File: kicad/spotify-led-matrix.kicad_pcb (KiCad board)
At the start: 2 copper layers, 101.5 x 128 mm, 73 parts, among them J1 +5V, J6 USB_C_Receptacle_USB2.0, Q1 IRLML6244TRPBF, Q10 IRLML6244TRPBF, Q2 SS8050-G, Q3 SS8050-G, Q4 IRLML6244TRPBF, Q5 IRLML6244TRPBF, Q6 IRLML6244TRPBF, Q7 IRLML6244TRPBF, Q8 IRLML6244TRPBF, Q9 IRLML6244TRPBF, SW1 SELECT, SW2 EN, SW3 BOOT, U1 ESP32-WROOM-32E, U2 5V_TO_3V3, U3 MC74HC1G14DTT1G, U6 MC74HC1G14DTT1G, U7 MC74HC1G14DTT1G, U8 FT234XD-R

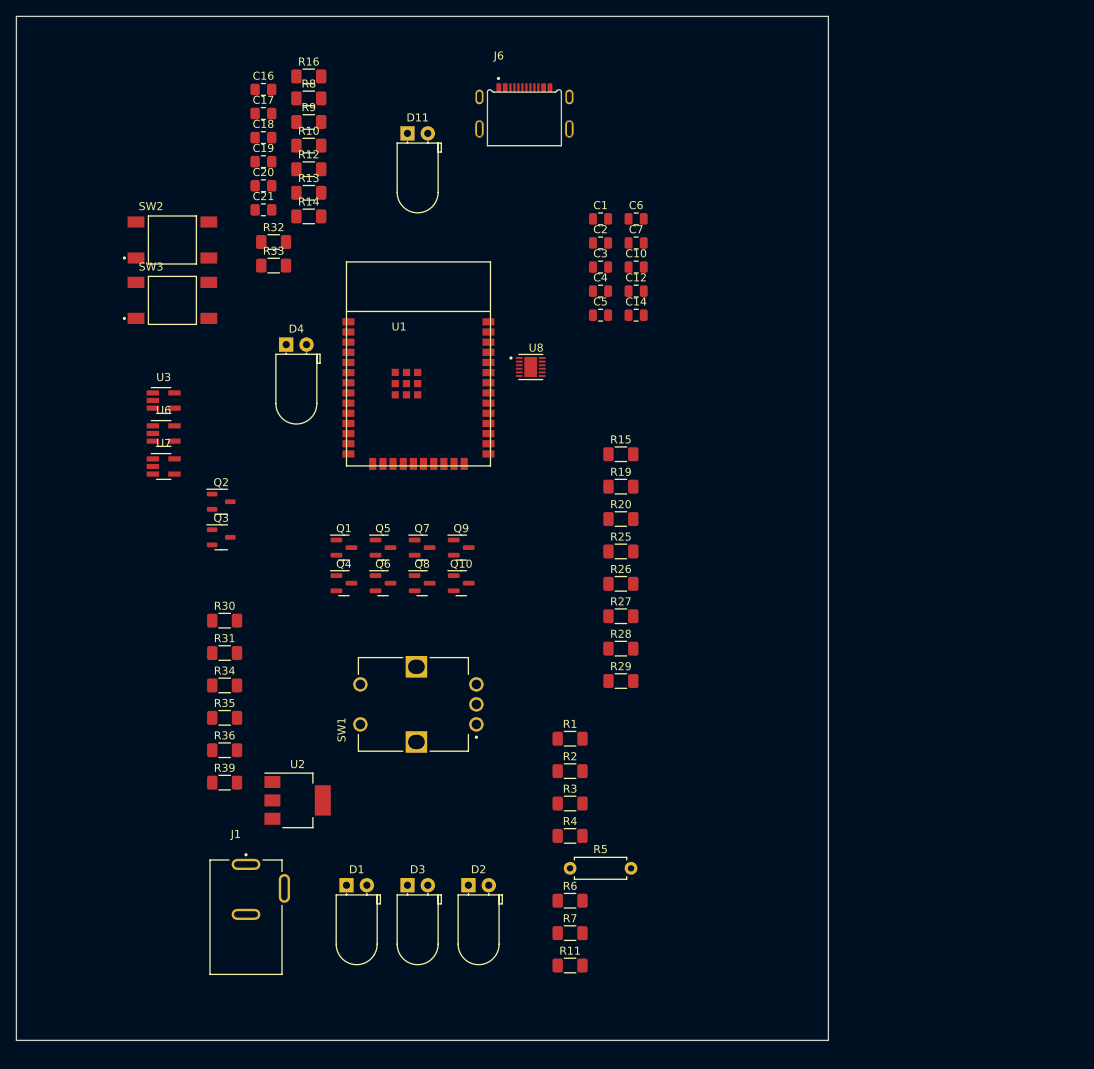
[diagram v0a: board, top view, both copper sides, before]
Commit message: Working out gitignore issues.
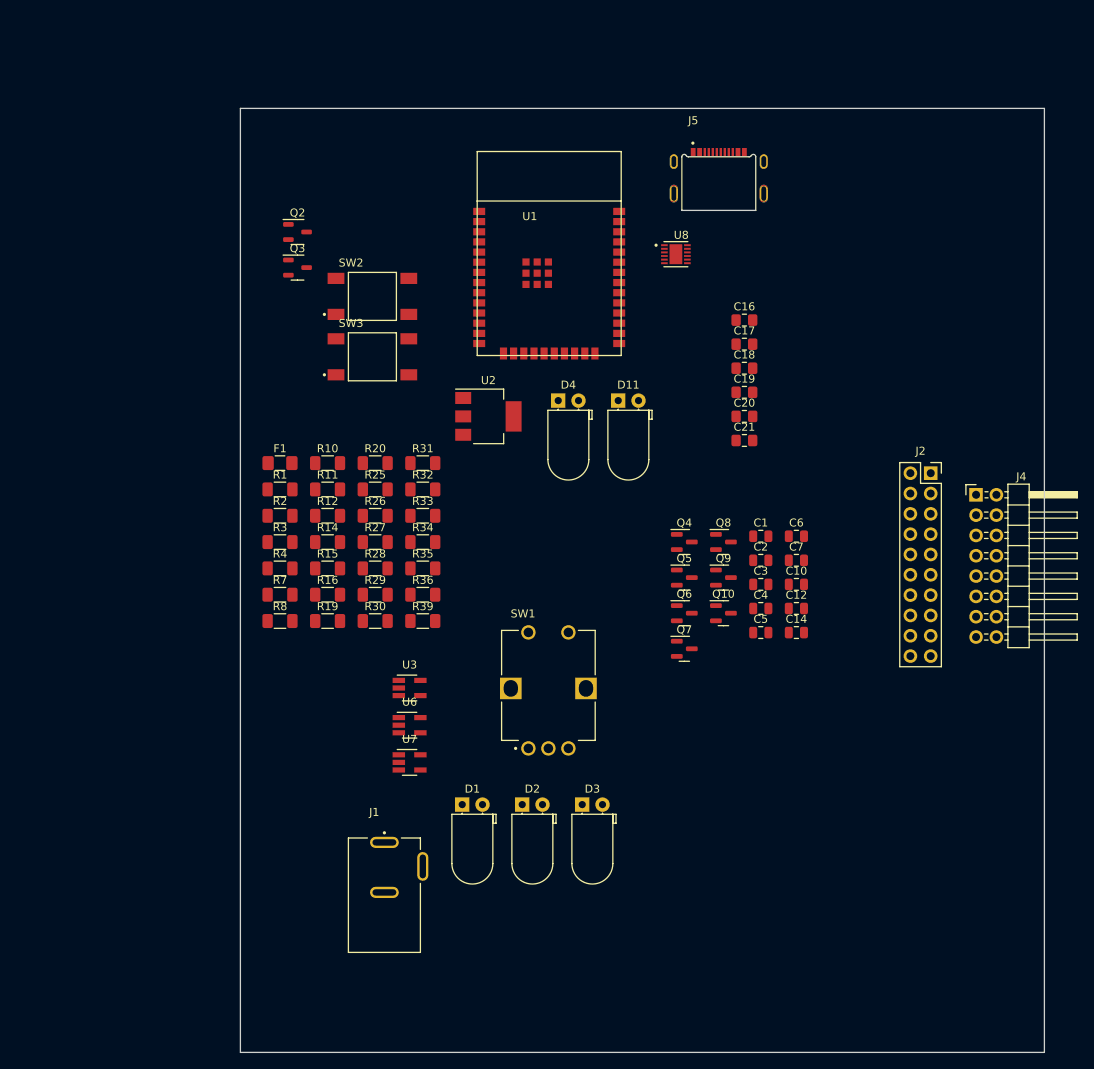
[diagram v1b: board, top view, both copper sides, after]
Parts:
- removed J6: USB_C_Receptacle_USB2.0, spotify-led-matrix:MOLEX_2169900003
- removed Q1: IRLML6244TRPBF, Package_TO_SOT_SMD:SOT-23
- removed R13, R9: 0, Resistor_SMD:R_1206_3216Metric_Pad1.30x1.75mm_HandSolder
- removed R5: 0, Resistor_THT:R_Axial_DIN0207_L6.3mm_D2.5mm_P7.62mm_Horizontal
- removed R6: 10k, Resistor_SMD:R_1206_3216Metric_Pad1.30x1.75mm_HandSolder
- added F1: Fuse, Fuse:Fuse_1206_3216Metric_Pad1.42x1.75mm_HandSolder, F.Cu at (120.0, 74.8)
- added J2: DSIPLAY_IN, Connector_PinSocket_2.54mm:PinSocket_2x10_P2.54mm_Vertical, F.Cu at (201.3, 76.1)
- added J4: DISPLAY_OUT, Connector_PinHeader_2.54mm:PinHeader_2x08_P2.54mm_Horizontal, F.Cu at (207.0, 78.8)
- added J5: USB_C_Receptacle_USB2.0, spotify-led-matrix:MOLEX_2169900003, F.Cu at (174.8, 41.1)
- SW1: value SELECT -> MODE_SELECT
- moved R11 66.8 mm to (125.9, 78.1)
- moved C16 66.7 mm to (178.0, 57.0)
- moved C17 66.7 mm to (178.0, 60.0)
- moved C18 66.7 mm to (178.0, 63.0)
- moved C19 66.7 mm to (178.0, 66.0)
- moved C20 66.7 mm to (178.0, 69.0)
- moved C21 66.7 mm to (178.0, 72.0)
- moved R8 65.4 mm to (120.0, 94.6)
- moved R16 64.8 mm to (125.9, 91.3)
- moved R7 55.7 mm to (120.0, 91.3)
- moved U2 53.6 mm to (146.0, 69.0)
- moved R4 49.3 mm to (120.0, 88.0)
- moved R3 48.8 mm to (120.0, 84.7)
- moved R2 48.3 mm to (120.0, 81.4)
- moved U7 48.1 mm to (136.2, 112.2)
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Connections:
- C10 pad 1: Net-(C10-Pad1) -> /BOOT_SW
- C6 pad 1: Net-(C6-Pad1) -> /EN_SW
- Q4 pad 3: /SELECT -> /MODE_SELECT
- R12 pad 2: /EN_BTN -> /EN_SW
- R30 pad 1: /SELECT -> /MODE_SELECT
- R8 pad 2: /BOOT_BTN -> /BOOT_SW
- SW1 pad P1: (no net) -> unconnected-(SW1-PadP1)
- SW1 pad P2: (no net) -> unconnected-(SW1-PadP2)
- SW2 pad 2: Net-(C6-Pad1) -> /EN_SW
- SW3 pad 2: Net-(C10-Pad1) -> /BOOT_SW
- U1 pad 10: unconnected-(U1-IO25-Pad10) -> /ROTARY_B
- U1 pad 11: unconnected-(U1-IO26-Pad11) -> /ROTARY_A
- U1 pad 13: /TMS -> /CLK
- U1 pad 14: /CLK -> unconnected-(U1-IO12-Pad14)
- U1 pad 26: unconnected-(U1-IO4-Pad26) -> /VOLUME
- U1 pad 28: unconnected-(U1-IO17-Pad28) -> /BRIGHTNESS
- U1 pad 33: unconnected-(U1-IO21-Pad33) -> /MODES
- U1 pad 9: unconnected-(U1-IO33-Pad9) -> /MODE_SELECT
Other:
- board size 101.5 x 128 mm -> 100.5 x 118 mm
